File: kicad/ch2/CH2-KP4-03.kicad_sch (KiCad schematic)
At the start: 7 parts

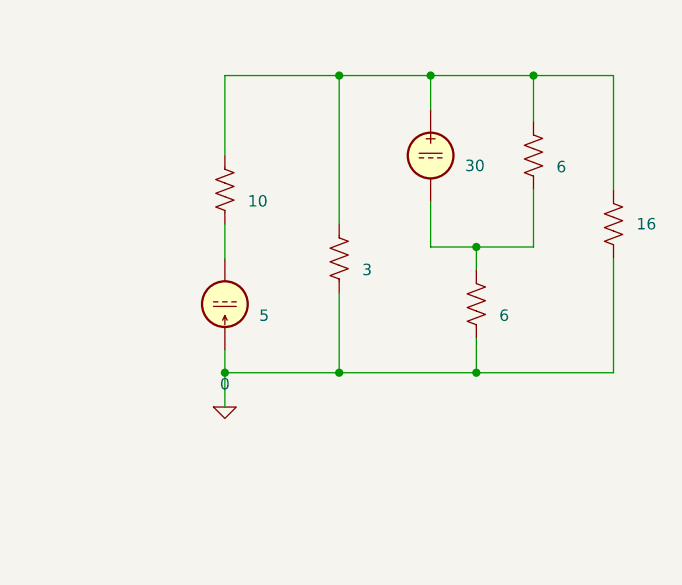
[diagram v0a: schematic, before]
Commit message: regular
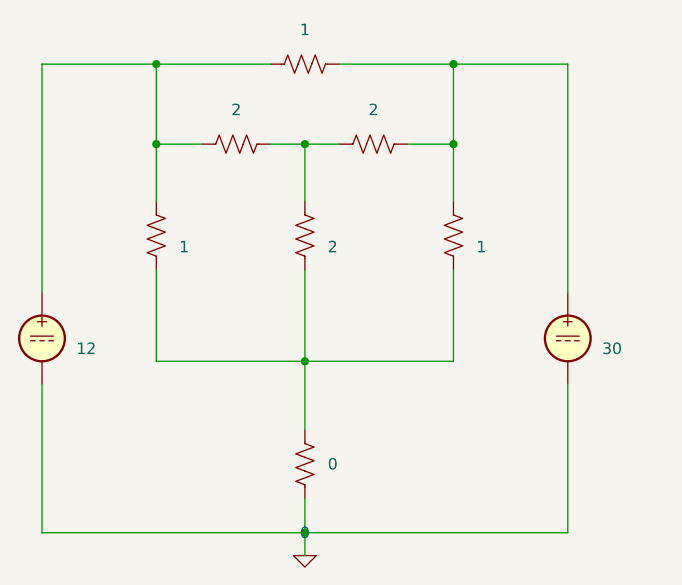
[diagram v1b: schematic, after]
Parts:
- removed I6: 5, symbol Simulation_SPICE:IDC
- removed R29: 10, symbol Device:R_US
- removed R30: 3, symbol Device:R_US
- removed R31, R32: 6, symbol Device:R_US
- removed R33: 16, symbol Device:R_US
- removed V12: 30, symbol Simulation_SPICE:VDC
- added R39: 0, symbol Device:R_US
- added R40, R41, R42: 1, symbol Device:R_US
- added R43, R44, R45: 2, symbol Device:R_US
- added V15: 12, symbol Simulation_SPICE:VDC
- added V16: 30, symbol Simulation_SPICE:VDC
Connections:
- net 0: now also R39.1, V15.2, V16.2
- new net: R39.2, R41.1, R42.1, R45.1
- new net: R40.2, R42.2, R44.1, V16.1
- new net: R43.1, R44.2, R45.2
- new net: R40.1, R41.2, R43.2, V15.1
